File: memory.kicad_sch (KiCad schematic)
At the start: 6 parts, among them J7 SD_Card_Receptacle, U5 M24C64-WMN6TP, U9 WE-TVS-824015043

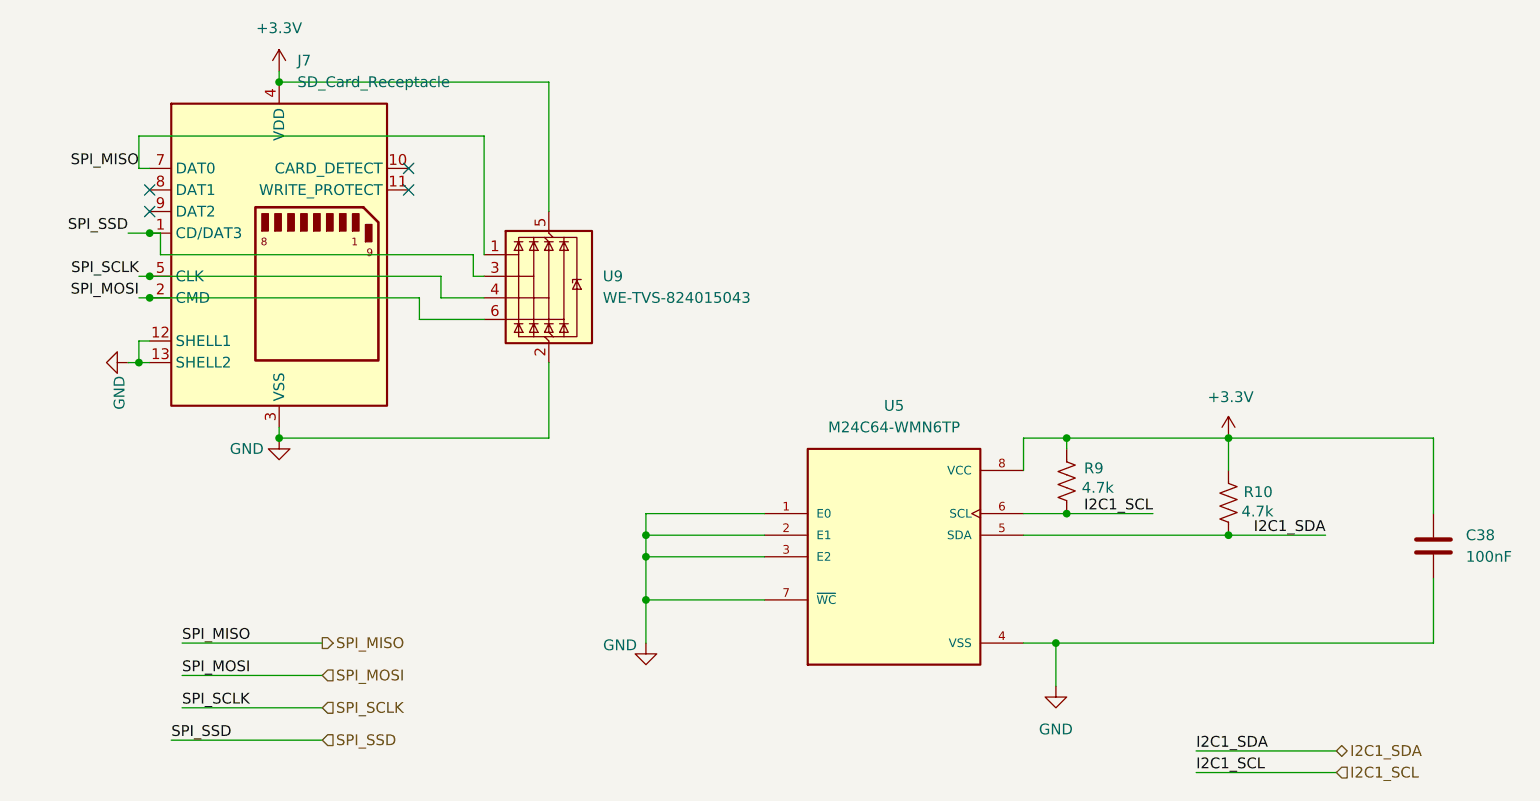
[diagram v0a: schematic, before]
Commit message: plane and jumper fix
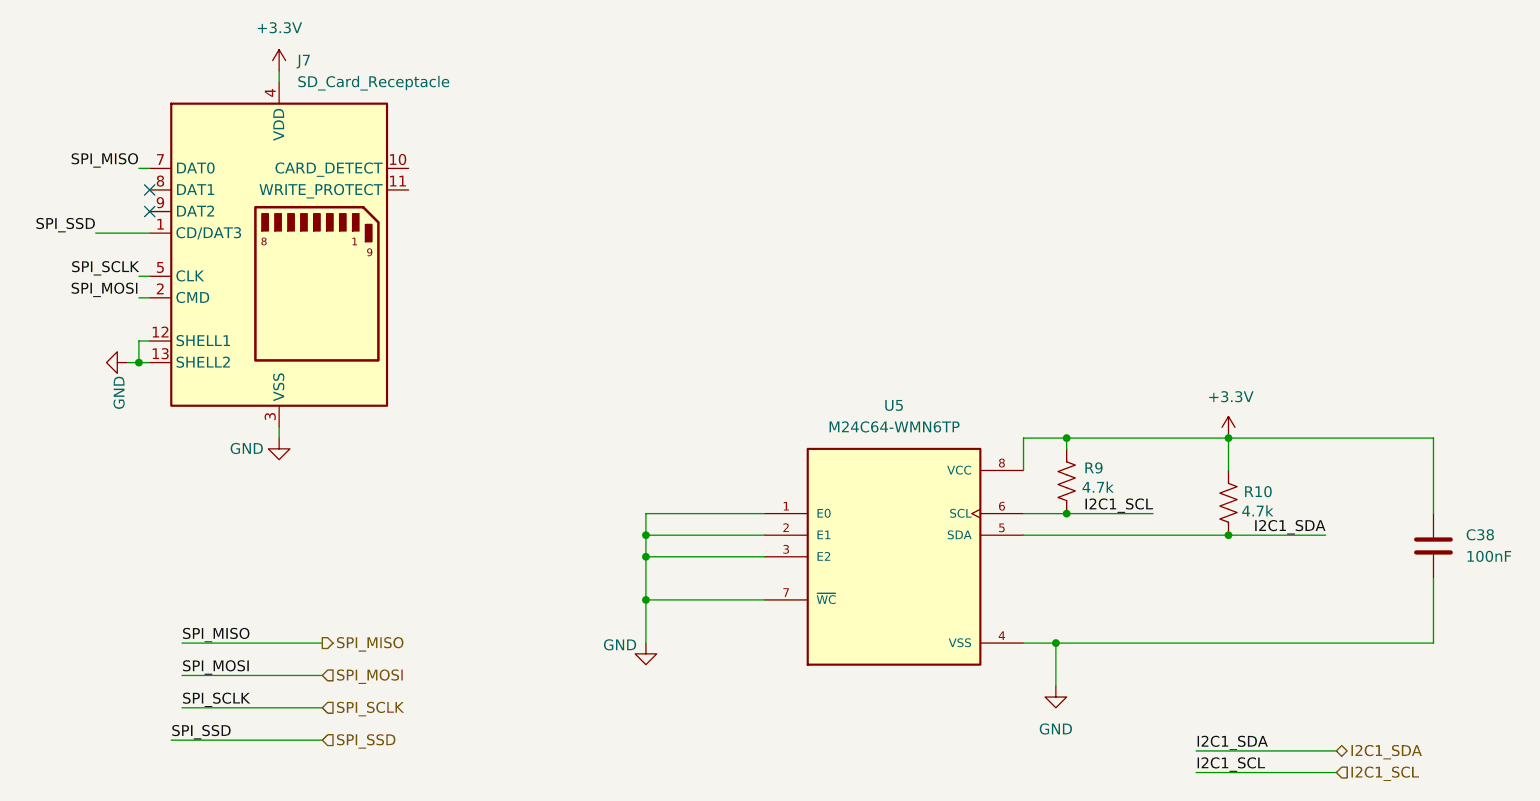
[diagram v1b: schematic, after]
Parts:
- removed U9: WE-TVS-824015043, Package_TO_SOT_SMD:SOT-23-6, symbol Power_Protection:WE-TVS-824015043
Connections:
- no-connect marks 4 -> 2
